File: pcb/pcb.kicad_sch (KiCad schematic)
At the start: 44 parts, among them J1 ICSP, J2 Debug 1, J3 Debug 2, P1 Power, Q1 Q_NPN_BCE, SW1 START, SW2 RESET, U1 PIC16F18346-P, U2 74HC595, U3 SCORE 1, U4 74HC595, U5 SCORE 2, U6 SSD1306

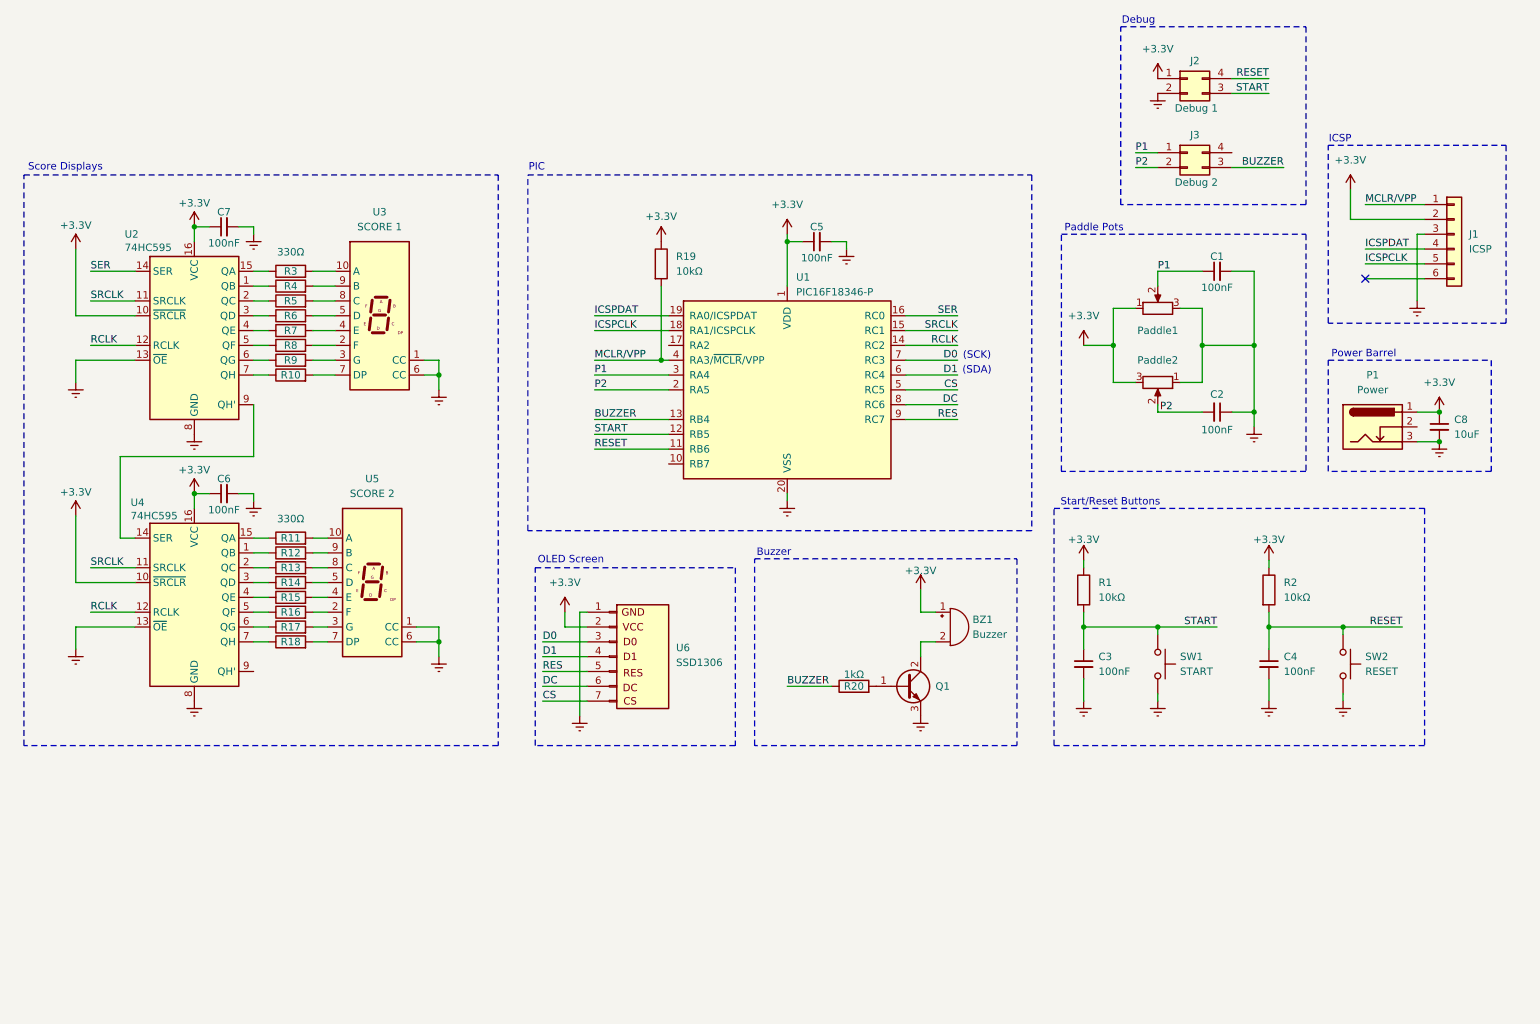
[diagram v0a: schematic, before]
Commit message: Layout PCB
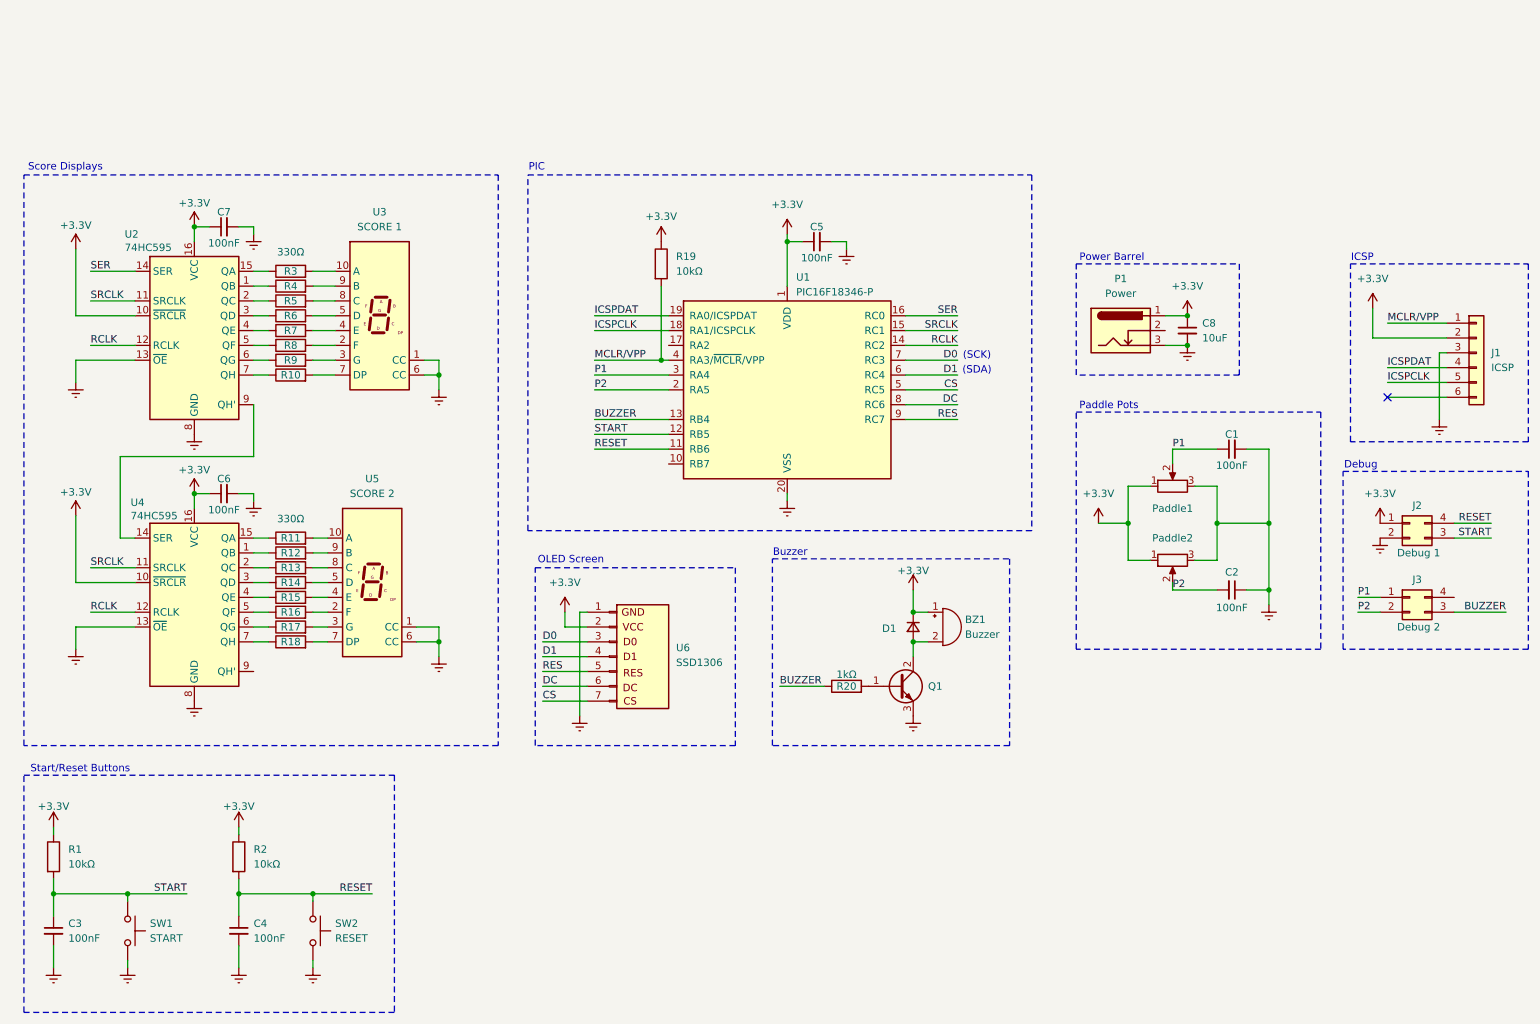
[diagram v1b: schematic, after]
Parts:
- added D1: D_Small, Diode_THT:D_DO-35_SOD27_P7.62mm_Horizontal, symbol Device:D_Small
- U2, U4: footprint Package_DIP:DIP-16_W7.62mm_LongPads -> Package_DIP:DIP-16_W7.62mm_Socket_LongPads
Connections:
- net +3.3V: now also Paddle2.1, D1.1 (K); no longer Paddle2.3
- net Earth: now also Paddle2.3; no longer Paddle2.1
- net at BZ1.2 (-), Q1.2 (C): now also D1.2 (A)
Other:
- moved on the sheet: BZ1, C1, C2, C3, C4, C8, J1, J2, J3, P1, Paddle1, Paddle2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
